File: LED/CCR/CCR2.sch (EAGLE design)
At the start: 6 parts, among them X2 MKDSN1,5/2-5,08, X3 MKDSN1,5/2-5,08

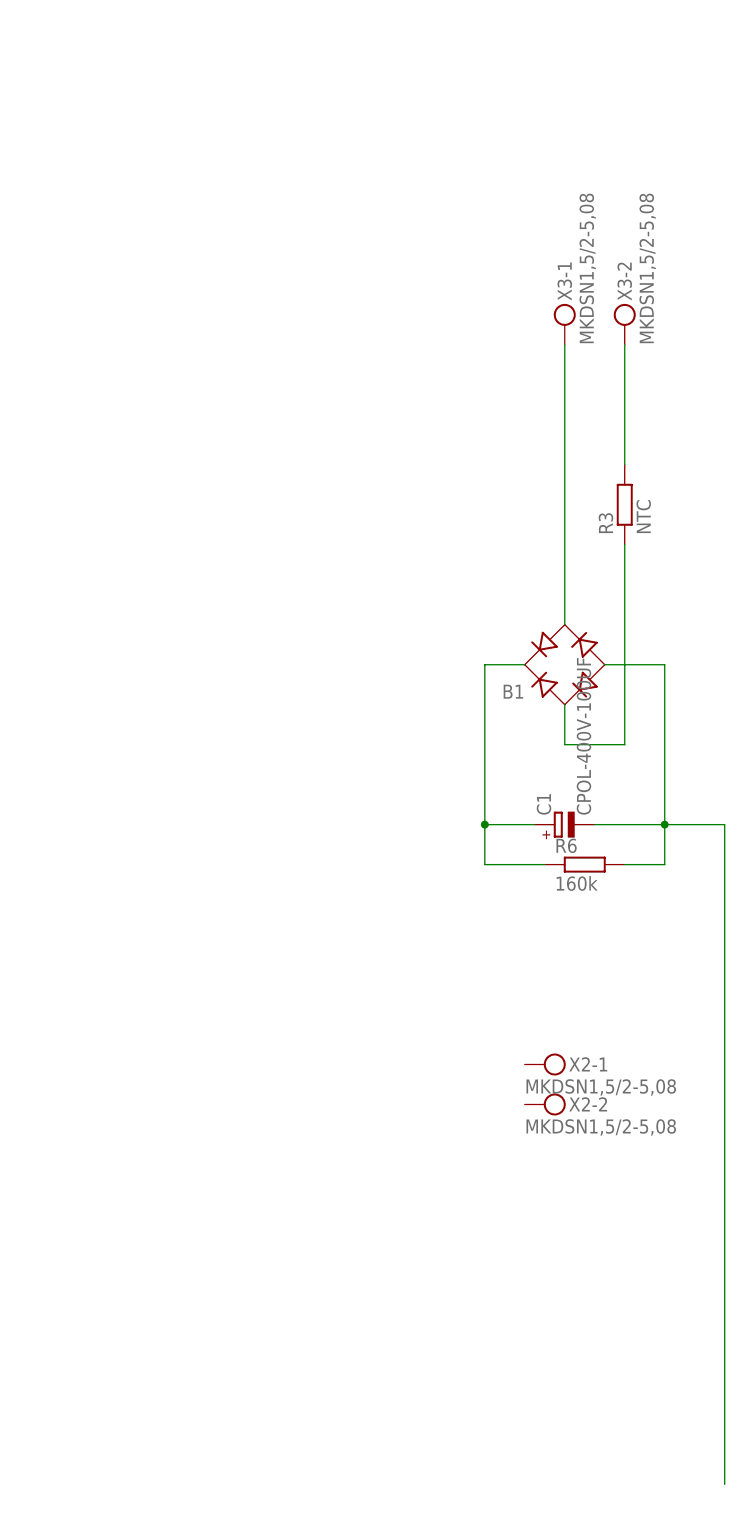
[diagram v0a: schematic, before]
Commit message: !
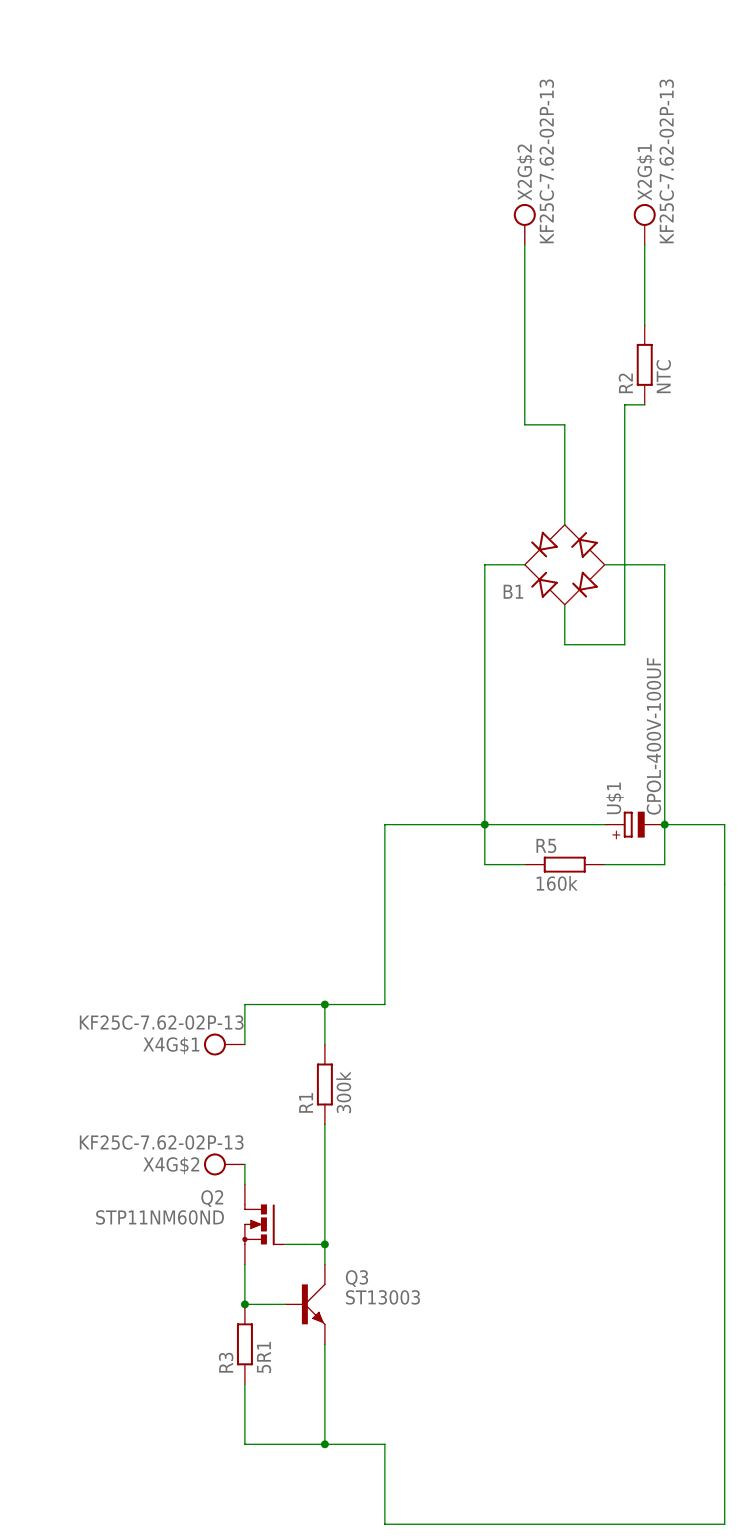
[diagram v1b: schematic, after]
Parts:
- removed C1: CPOL-400V-100UF, Namenlos:CPOL-400V-100UF
- removed R6: 160k, rcl:R-EU_0204/7
- removed X3: MKDSN1,5/2-5,08, con-phoenix-508:MKDSN1,5/2-5,08
- added Q2: STP11NM60ND, transistor-power:BUZ11BV
- added Q3: ST13003, Namenlos:KSP42TA
- added R1: 300k, rcl:R-EU_0411/12
- added R2: NTC, rcl:R-EU_0309/10
- added R5: 160k, rcl:R-EU_0204/7
- added U$1: CPOL-400V-100UF, Namenlos:CPOL-400V-100UF
- added X4: KF25C-7.62-02P-13, Namenlos:KF25C-7.62-02P-13
- R3: value NTC -> 5R1; device rcl:R-EU_0309/10 -> rcl:R-EU_R0805
- X2: value MKDSN1,5/2-5,08 -> KF25C-7.62-02P-13; device con-phoenix-508:MKDSN1,5/2-5,08 -> Namenlos:KF25C-7.62-02P-13
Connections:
- removed net GND: B1.-, C1.-, R6.2
- removed net N$11: B1.AC1, R3.1
- new net N$3: R2.2, X2G$1.KL
- new net N$4: B1.AC2, X2G$2.KL
- new net N$6: Q2.S, Q3.B, R3.2
- new net N$7: Q2.G, Q3.C, R1.1
- new net N$9: B1.-, Q3.E, R3.1, R5.2, U$1.-
- net N$1: now also R1.2, R5.1, U$1.+, X4G$1.KL; no longer C1.+, R6.1
- net N$2: now also B1.AC1, R2.1; no longer R3.2, X3-2.KL
- net N$5: now also Q2.D, X4G$2.KL; no longer B1.AC2, X3-1.KL
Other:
- moved on the sheet: B1, R3
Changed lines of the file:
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@@
 </classes>
 <parts>
-<part name="X2" library="con-phoenix-508" deviceset="MKDSN1,5/2-5,08" device=""/>
+<part name="R1" library="rcl" deviceset="R-EU_" device="0411/12" value="300k"/>
+<part name="R3" library="rcl" deviceset="R-EU_" device="R0805" value="5R1"/>
+<part name="Q2" library="transistor-power" deviceset="BUZ11" device="BV" value="STP11NM60ND"/>
+<part name="Q3" library="Namenlos" deviceset="KSP42TA" device="" value="ST13003"/>
 <part name="B1" library="rectifier" deviceset="RB1A" device=""/>
-<part name="C1" library="Namenlos" deviceset="CPOL-400V-100UF" device=""/>
-<part name="R6" library="rcl" deviceset="R-EU_" device="0204/7" value="160k"/>
-<part name="X3" library="con-phoenix-508" deviceset="MKDSN1,5/2-5,08" device=""/>
-<part name="R3" library="rcl" deviceset="R-EU_" device="0309/10" value="NTC"/>
+<part name="R5" library="rcl" deviceset="R-EU_" device="0204/7" value="160k"/>
+<part name="R2" library="rcl" deviceset="R-EU_" device="0309/10" value="NTC"/>
+<part name="U$1" library="Namenlos" deviceset="CPOL-400V-100UF" device=""/>
+<part name="X2" library="Namenlos" deviceset="KF25C-7.62-02P-13" device=""/>
+<part name="X4" library="Namenlos" deviceset="KF25C-7.62-02P-13" device=""/>
 </parts>
 <sheets>
@@
 </plain>
 <instances>
-<instance part="X2" gate="-1" x="66.04" y="71.12"/>
-<instance part="X2" gate="-2" x="66.04" y="66.04"/>
-<instance part="B1" gate="1" x="68.58" y="121.92" rot="R180"/>
-<instance part="C1" gate="G$1" x="68.58" y="101.6" rot="R90"/>
-<instance part="R6" gate="G$1" x="71.12" y="96.52"/>
-<instance part="X3" gate="-1" x="68.58" y="165.1" rot="R90"/>
-<instance part="X3" gate="-2" x="76.2" y="165.1" rot="R90"/>
-<instance part="R3" gate="G$1" x="76.2" y="142.24" rot="R90"/>
+<instance part="R1" gate="G$1" x="38.1" y="68.58" rot="R90"/>
+<instance part="R3" gate="G$1" x="27.94" y="35.56" rot="R90"/>
+<instance part="Q2" gate="1" x="30.48" y="50.8" rot="MR0"/>
+<instance part="Q3" gate="G$1" x="35.56" y="40.64"/>
+<instance part="B1" gate="1" x="68.58" y="134.62" rot="R180"/>
+<instance part="R5" gate="G$1" x="68.58" y="96.52"/>
+<instance part="R2" gate="G$1" x="78.74" y="160.02" rot="R90"/>
+<instance part="U$1" gate="G$1" x="77.47" y="101.6" rot="R90"/>
+<instance part="X2" gate="G$1" x="78.74" y="175.26" rot="R90"/>
+<instance part="X2" gate="G$2" x="63.5" y="175.26" rot="R90"/>
+<instance part="X4" gate="G$1" x="27.94" y="73.66" rot="R180"/>
+<instance part="X4" gate="G$2" x="27.94" y="58.42" rot="R180"/>
 </instances>
 <busses>
@@
 <net name="N$1" class="0">
 <segment>
-<pinref part="C1" gate="G$1" pin="+"/>
+<pinref part="R1" gate="G$1" pin="2"/>
+<wire x1="45.72" y1="78.74" x2="38.1" y2="78.74" width="0.1524" layer="91"/>
+<wire x1="38.1" y1="78.74" x2="38.1" y2="73.66" width="0.1524" layer="91"/>
+<wire x1="27.94" y1="73.66" x2="27.94" y2="78.74" width="0.1524" layer="91"/>
+<wire x1="27.94" y1="78.74" x2="38.1" y2="78.74" width="0.1524" layer="91"/>
+<junction x="38.1" y="78.74"/>
+<wire x1="45.72" y1="78.74" x2="45.72" y2="101.6" width="0.1524" layer="91"/>
+<wire x1="45.72" y1="101.6" x2="58.42" y2="101.6" width="0.1524" layer="91"/>
 <pinref part="B1" gate="1" pin="+"/>
-<wire x1="58.42" y1="101.6" x2="64.77" y2="101.6" width="0.1524" layer="91"/>
-<wire x1="63.5" y1="121.92" x2="58.42" y2="121.92" width="0.1524" layer="91"/>
-<wire x1="58.42" y1="121.92" x2="58.42" y2="101.6" width="0.1524" layer="91"/>
+<wire x1="63.5" y1="134.62" x2="58.42" y2="134.62" width="0.1524" layer="91"/>
+<wire x1="58.42" y1="134.62" x2="58.42" y2="101.6" width="0.1524" layer="91"/>
 <junction x="58.42" y="101.6"/>
-<wire x1="58.42" y1="96.52" x2="58.42" y2="101.6" width="0.1524" layer="91"/>
-<pinref part="R6" gate="G$1" pin="1"/>
-<wire x1="58.42" y1="96.52" x2="66.04" y2="96.52" width="0.1524" layer="91"/>
+<wire x1="58.42" y1="101.6" x2="58.42" y2="96.52" width="0.1524" layer="91"/>
+<pinref part="R5" gate="G$1" pin="1"/>
+<wire x1="58.42" y1="96.52" x2="63.5" y2="96.52" width="0.1524" layer="91"/>
+<pinref part="U$1" gate="G$1" pin="+"/>
+<wire x1="73.66" y1="101.6" x2="58.42" y2="101.6" width="0.1524" layer="91"/>
+<pinref part="X4" gate="G$1" pin="KL"/>
 </segment>
 </net>
-<net name="GND" class="0">
+<net name="N$5" class="0">
 <segment>
-<wire x1="88.9" y1="17.78" x2="88.9" y2="101.6" width="0.1524" layer="91"/>
-<pinref part="C1" gate="G$1" pin="-"/>
-<wire x1="72.39" y1="101.6" x2="81.28" y2="101.6" width="0.1524" layer="91"/>
-<wire x1="81.28" y1="101.6" x2="88.9" y2="101.6" width="0.1524" layer="91"/>
-<pinref part="B1" gate="1" pin="-"/>
-<wire x1="73.66" y1="121.92" x2="81.28" y2="121.92" width="0.1524" layer="91"/>
-<wire x1="81.28" y1="121.92" x2="81.28" y2="101.6" width="0.1524" layer="91"/>
-<junction x="81.28" y="101.6"/>
-<pinref part="R6" gate="G$1" pin="2"/>
-<wire x1="76.2" y1="96.52" x2="81.28" y2="96.52" width="0.1524" layer="91"/>
-<wire x1="81.28" y1="96.52" x2="81.28" y2="101.6" width="0.1524" layer="91"/>
+<pinref part="Q2" gate="1" pin="D"/>
+<wire x1="27.94" y1="58.42" x2="27.94" y2="55.88" width="0.1524" layer="91"/>
+<pinref part="X4" gate="G$2" pin="KL"/>
 </segment>
 </net>
-<net name="N$11" class="0">
+<net name="N$6" class="0">
 <segment>
-<pinref part="B1" gate="1" pin="AC1"/>
-<wire x1="76.2" y1="111.76" x2="68.58" y2="111.76" width="0.1524" layer="91"/>
-<wire x1="68.58" y1="111.76" x2="68.58" y2="116.84" width="0.1524" layer="91"/>
+<pinref part="R3" gate="G$1" pin="2"/>
+<wire x1="27.94" y1="45.72" x2="27.94" y2="40.64" width="0.1524" layer="91"/>
+<pinref part="Q2" gate="1" pin="S"/>
+<pinref part="Q3" gate="G$1" pin="B"/>
+<wire x1="33.02" y1="40.64" x2="27.94" y2="40.64" width="0.1524" layer="91"/>
+<junction x="27.94" y="40.64"/>
+</segment>
+</net>
+<net name="N$7" class="0">
+<segment>
+<wire x1="38.1" y1="48.26" x2="35.56" y2="48.26" width="0.1524" layer="91"/>
+<pinref part="R1" gate="G$1" pin="1"/>
+<wire x1="38.1" y1="63.5" x2="38.1" y2="48.26" width="0.1524" layer="91"/>
+<pinref part="Q2" gate="1" pin="G"/>
+<wire x1="33.02" y1="48.26" x2="35.56" y2="48.26" width="0.1524" layer="91"/>
+<pinref part="Q3" gate="G$1" pin="C"/>
+<wire x1="38.1" y1="45.72" x2="38.1" y2="48.26" width="0.1524" layer="91"/>
+<junction x="38.1" y="48.26"/>
+</segment>
+</net>
+<net name="N$9" class="0">
+<segment>
 <pinref part="R3" gate="G$1" pin="1"/>
-<wire x1="76.2" y1="111.76" x2="76.2" y2="137.16" width="0.1524" layer="91"/>
+<wire x1="27.94" y1="30.48" x2="27.94" y2="22.86" width="0.1524" layer="91"/>
+<wire x1="27.94" y1="22.86" x2="38.1" y2="22.86" width="0.1524" layer="91"/>
+<wire x1="38.1" y1="22.86" x2="45.72" y2="22.86" width="0.1524" layer="91"/>
+<wire x1="38.1" y1="35.56" x2="38.1" y2="22.86" width="0.1524" layer="91"/>
+<junction x="38.1" y="22.86"/>
+<pinref part="Q3" gate="G$1" pin="E"/>
+<wire x1="45.72" y1="22.86" x2="45.72" y2="12.7" width="0.1524" layer="91"/>
+<wire x1="45.72" y1="12.7" x2="88.9" y2="12.7" width="0.1524" layer="91"/>
+<wire x1="88.9" y1="12.7" x2="88.9" y2="93.98" width="0.1524" layer="91"/>
+<wire x1="81.28" y1="101.6" x2="88.9" y2="101.6" width="0.1524" layer="91"/>
+<wire x1="88.9" y1="101.6" x2="88.9" y2="93.98" width="0.1524" layer="91"/>
+<pinref part="B1" gate="1" pin="-"/>
+<wire x1="73.66" y1="134.62" x2="81.28" y2="134.62" width="0.1524" layer="91"/>
+<wire x1="81.28" y1="134.62" x2="81.28" y2="101.6" width="0.1524" layer="91"/>
+<junction x="81.28" y="101.6"/>
+<pinref part="R5" gate="G$1" pin="2"/>
+<wire x1="73.66" y1="96.52" x2="81.28" y2="96.52" width="0.1524" layer="91"/>
+<wire x1="81.28" y1="96.52" x2="81.28" y2="101.6" width="0.1524" layer="91"/>
+<pinref part="U$1" gate="G$1" pin="-"/>
+</segment>
+</net>
+<net name="N$4" class="0">
+<segment>
+<wire x1="63.5" y1="175.26" x2="63.5" y2="152.4" width="0.1524" layer="91"/>
+<pinref part="B1" gate="1" pin="AC2"/>
+<wire x1="63.5" y1="152.4" x2="68.58" y2="152.4" width="0.1524" layer="91"/>
+<wire x1="68.58" y1="152.4" x2="68.58" y2="139.7" width="0.1524" layer="91"/>
+<pinref part="X2" gate="G$2" pin="KL"/>
 </segment>
 </net>
 <net name="N$2" class="0">
 <segment>
-<pinref part="X3" gate="-2" pin="KL"/>
-<pinref part="R3" gate="G$1" pin="2"/>
-<wire x1="76.2" y1="147.32" x2="76.2" y2="162.56" width="0.1524" layer="91"/>
+<pinref part="B1" gate="1" pin="AC1"/>
+<wire x1="68.58" y1="129.54" x2="68.58" y2="124.46" width="0.1524" layer="91"/>
+<wire x1="68.58" y1="124.46" x2="76.2" y2="124.46" width="0.1524" layer="91"/>
+<pinref part="R2" gate="G$1" pin="1"/>
+<wire x1="78.74" y1="154.94" x2="76.2" y2="154.94" width="0.1524" layer="91"/>
+<wire x1="76.2" y1="154.94" x2="76.2" y2="124.46" width="0.1524" layer="91"/>
 </segment>
 </net>
-<net name="N$5" class="0">
+<net name="N$3" class="0">
 <segment>
-<pinref part="X3" gate="-1" pin="KL"/>
-<pinref part="B1" gate="1" pin="AC2"/>
-<wire x1="68.58" y1="162.56" x2="68.58" y2="127" width="0.1524" layer="91"/>
+<pinref part="R2" gate="G$1" pin="2"/>
+<wire x1="78.74" y1="175.26" x2="78.74" y2="165.1" width="0.1524" layer="91"/>
+<pinref part="X2" gate="G$1" pin="KL"/>
 </segment>
 </net>
